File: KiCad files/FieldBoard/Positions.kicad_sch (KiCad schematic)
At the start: 52 parts

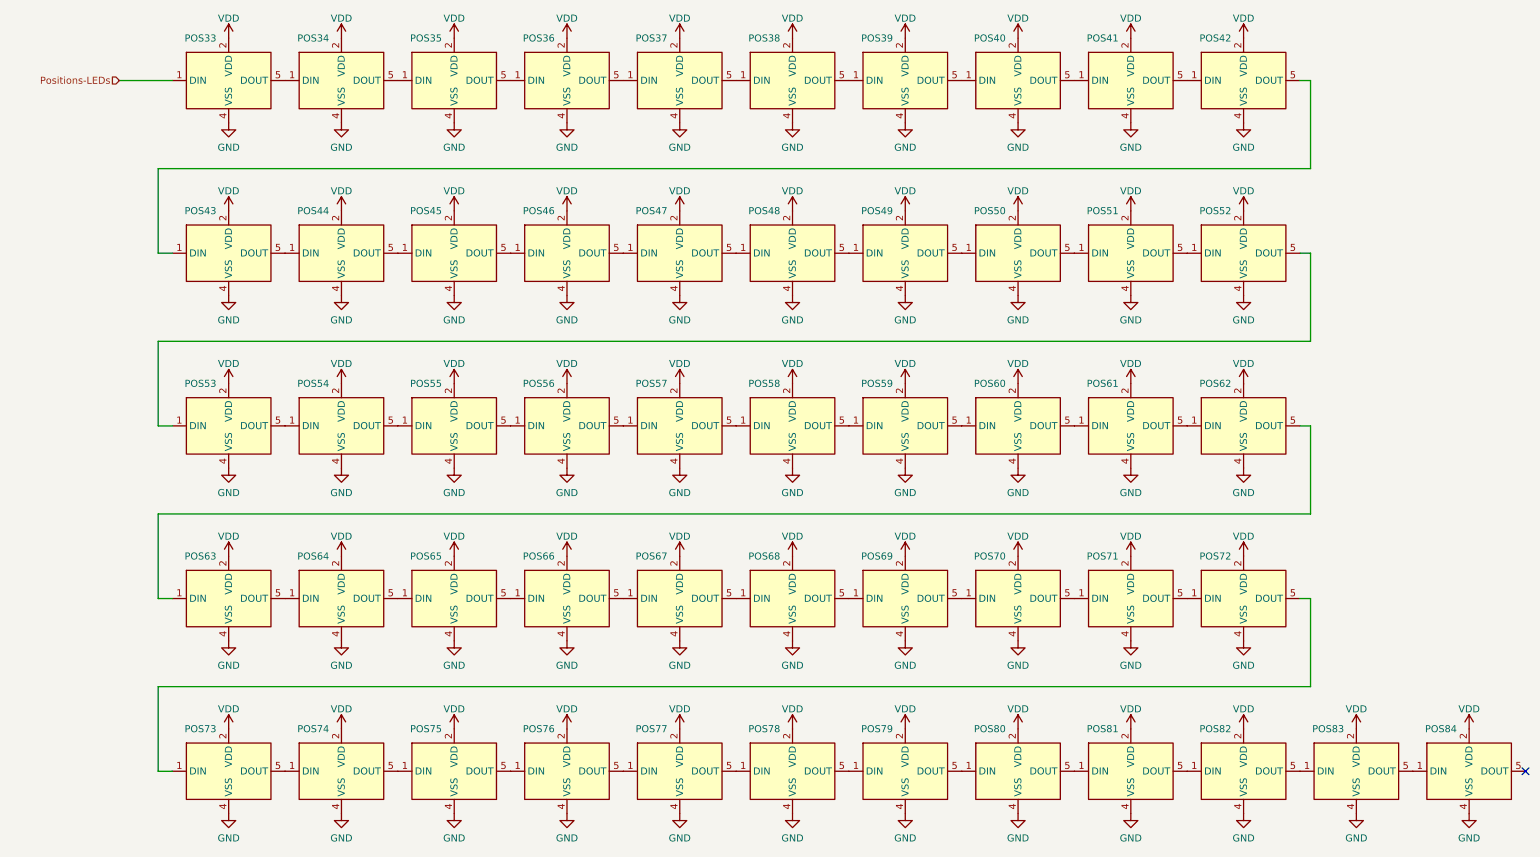
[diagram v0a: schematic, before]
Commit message: v2
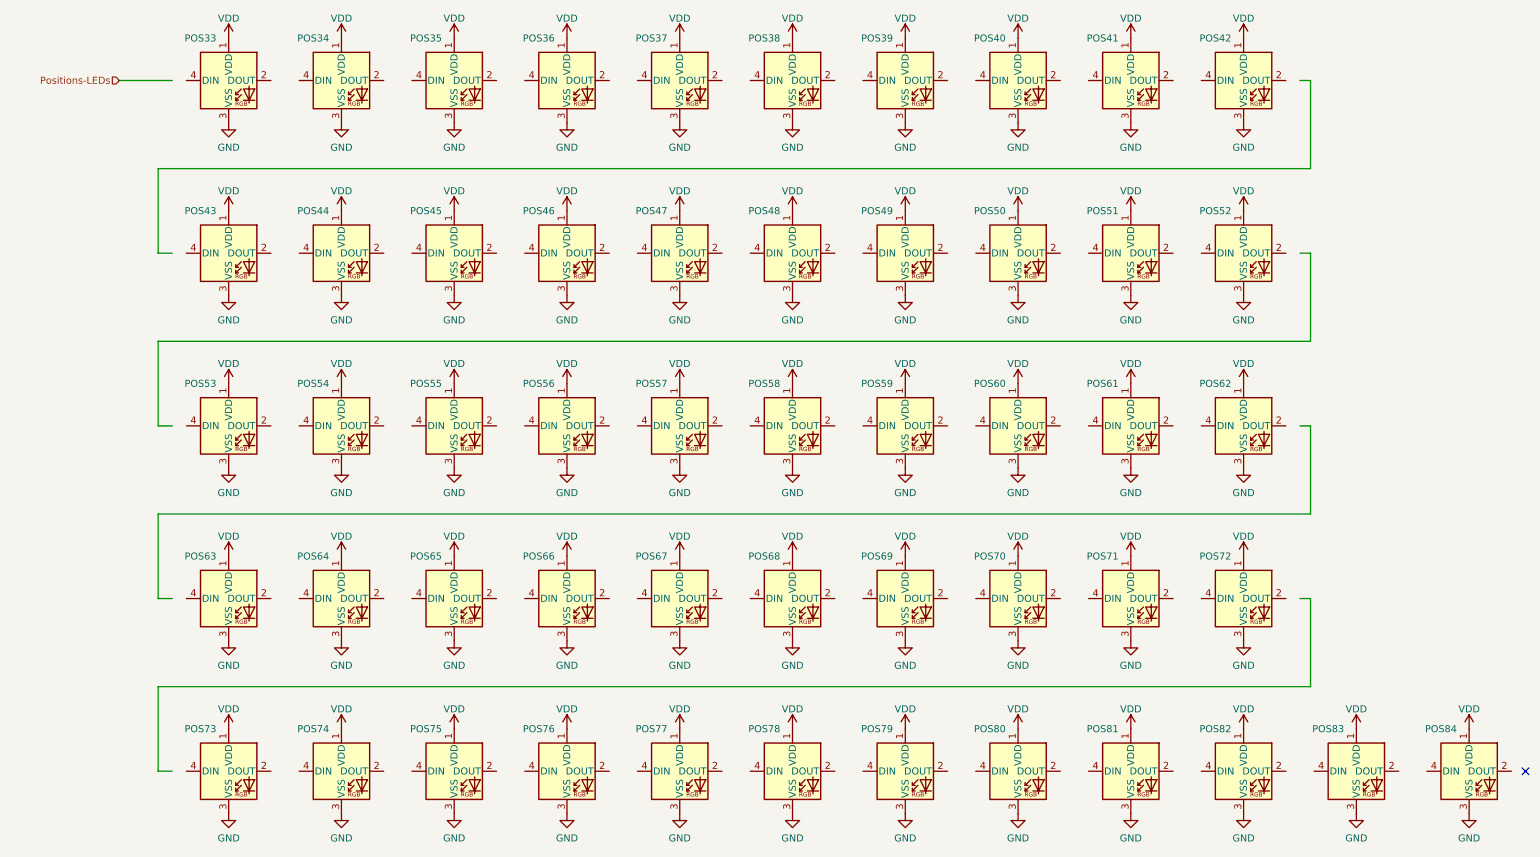
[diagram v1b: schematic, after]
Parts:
- POS33, POS34, POS35, POS36, POS37, POS38, POS39, POS40, POS41, POS42, POS43, POS44, POS45, POS46, POS47, POS48, POS49, POS50, POS51, POS52, POS53, POS54, POS55, POS56, POS57, POS58, POS59, POS60, POS61, POS62, POS63, POS64, POS65, POS66, POS67, POS68, POS69, POS70, POS71, POS72, POS73, POS74, POS75, POS76, POS77, POS78, POS79, POS80, POS81, POS82, POS83, POS84: footprint FieldBoard_footprint:WS2812-4020-dual-7mm_bezMaske -> LED_SMD:LED_WS2812B_PLCC4_5.0x5.0mm_P3.2mm; symbol FieldBoard_symbol:WS2812-4020_dual -> LED:WS2812B
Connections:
- net GND: now also POS33.3 (VSS), POS34.3 (VSS), POS35.3 (VSS), POS36.3 (VSS), POS37.3 (VSS), POS38.3 (VSS), POS39.3 (VSS), POS40.3 (VSS), POS41.3 (VSS), POS42.3 (VSS), POS43.3 (VSS), POS44.3 (VSS), POS45.3 (VSS), POS46.3 (VSS), POS47.3 (VSS), POS48.3 (VSS), POS49.3 (VSS), POS50.3 (VSS), POS51.3 (VSS), POS52.3 (VSS), POS53.3 (VSS), POS54.3 (VSS), POS55.3 (VSS), POS56.3 (VSS), POS57.3 (VSS), POS58.3 (VSS), POS59.3 (VSS), POS60.3 (VSS), POS61.3 (VSS), POS62.3 (VSS), POS63.3 (VSS), POS64.3 (VSS), POS65.3 (VSS), POS66.3 (VSS), POS67.3 (VSS), POS68.3 (VSS), POS69.3 (VSS), POS70.3 (VSS), POS71.3 (VSS), POS72.3 (VSS), POS73.3 (VSS), POS74.3 (VSS), POS75.3 (VSS), POS76.3 (VSS), POS77.3 (VSS), POS78.3 (VSS), POS79.3 (VSS), POS80.3 (VSS), POS81.3 (VSS), POS82.3 (VSS), POS83.3 (VSS), POS84.3 (VSS); no longer POS33.4 (VSS), POS34.4 (VSS), POS35.4 (VSS), POS36.4 (VSS), POS37.4 (VSS), POS38.4 (VSS), POS39.4 (VSS), POS40.4 (VSS), POS41.4 (VSS), POS42.4 (VSS), POS43.4 (VSS), POS44.4 (VSS), POS45.4 (VSS), POS46.4 (VSS), POS47.4 (VSS), POS48.4 (VSS), POS49.4 (VSS), POS50.4 (VSS), POS51.4 (VSS), POS52.4 (VSS), POS53.4 (VSS), POS54.4 (VSS), POS55.4 (VSS), POS56.4 (VSS), POS57.4 (VSS), POS58.4 (VSS), POS59.4 (VSS), POS60.4 (VSS), POS61.4 (VSS), POS62.4 (VSS), POS63.4 (VSS), POS64.4 (VSS), POS65.4 (VSS), POS66.4 (VSS), POS67.4 (VSS), POS68.4 (VSS), POS69.4 (VSS), POS70.4 (VSS), POS71.4 (VSS), POS72.4 (VSS), POS73.4 (VSS), POS74.4 (VSS), POS75.4 (VSS), POS76.4 (VSS), POS77.4 (VSS), POS78.4 (VSS), POS79.4 (VSS), POS80.4 (VSS), POS81.4 (VSS), POS82.4 (VSS), POS83.4 (VSS), POS84.4 (VSS)
- net Positions-LEDs: no longer POS33.1 (DIN)
- net VDD: now also POS33.1 (VDD), POS34.1 (VDD), POS35.1 (VDD), POS36.1 (VDD), POS37.1 (VDD), POS38.1 (VDD), POS39.1 (VDD), POS40.1 (VDD), POS41.1 (VDD), POS42.1 (VDD), POS43.1 (VDD), POS44.1 (VDD), POS45.1 (VDD), POS46.1 (VDD), POS47.1 (VDD), POS48.1 (VDD), POS49.1 (VDD), POS50.1 (VDD), POS51.1 (VDD), POS52.1 (VDD), POS53.1 (VDD), POS54.1 (VDD), POS55.1 (VDD), POS56.1 (VDD), POS57.1 (VDD), POS58.1 (VDD), POS59.1 (VDD), POS60.1 (VDD), POS61.1 (VDD), POS62.1 (VDD), POS63.1 (VDD), POS64.1 (VDD), POS65.1 (VDD), POS66.1 (VDD), POS67.1 (VDD), POS68.1 (VDD), POS69.1 (VDD), POS70.1 (VDD), POS71.1 (VDD), POS72.1 (VDD), POS73.1 (VDD), POS74.1 (VDD), POS75.1 (VDD), POS76.1 (VDD), POS77.1 (VDD), POS78.1 (VDD), POS79.1 (VDD), POS80.1 (VDD), POS81.1 (VDD), POS82.1 (VDD), POS83.1 (VDD), POS84.1 (VDD); no longer POS33.2 (VDD), POS34.2 (VDD), POS35.2 (VDD), POS36.2 (VDD), POS37.2 (VDD), POS38.2 (VDD), POS39.2 (VDD), POS40.2 (VDD), POS41.2 (VDD), POS42.2 (VDD), POS43.2 (VDD), POS44.2 (VDD), POS45.2 (VDD), POS46.2 (VDD), POS47.2 (VDD), POS48.2 (VDD), POS49.2 (VDD), POS50.2 (VDD), POS51.2 (VDD), POS52.2 (VDD), POS53.2 (VDD), POS54.2 (VDD), POS55.2 (VDD), POS56.2 (VDD), POS57.2 (VDD), POS58.2 (VDD), POS59.2 (VDD), POS60.2 (VDD), POS61.2 (VDD), POS62.2 (VDD), POS63.2 (VDD), POS64.2 (VDD), POS65.2 (VDD), POS66.2 (VDD), POS67.2 (VDD), POS68.2 (VDD), POS69.2 (VDD), POS70.2 (VDD), POS71.2 (VDD), POS72.2 (VDD), POS73.2 (VDD), POS74.2 (VDD), POS75.2 (VDD), POS76.2 (VDD), POS77.2 (VDD), POS78.2 (VDD), POS79.2 (VDD), POS80.2 (VDD), POS81.2 (VDD), POS82.2 (VDD), POS83.2 (VDD), POS84.2 (VDD)
